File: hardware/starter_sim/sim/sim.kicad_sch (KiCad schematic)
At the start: 22 parts, among them M1 Motor_DC, Q1 AO3400A, Q2 AO3400A, Q3 AO3401A, Q4 AO3400A, Q5 AO3401A, Q6 AO3400A, Q7 AO3401A, Q8 AO3401A

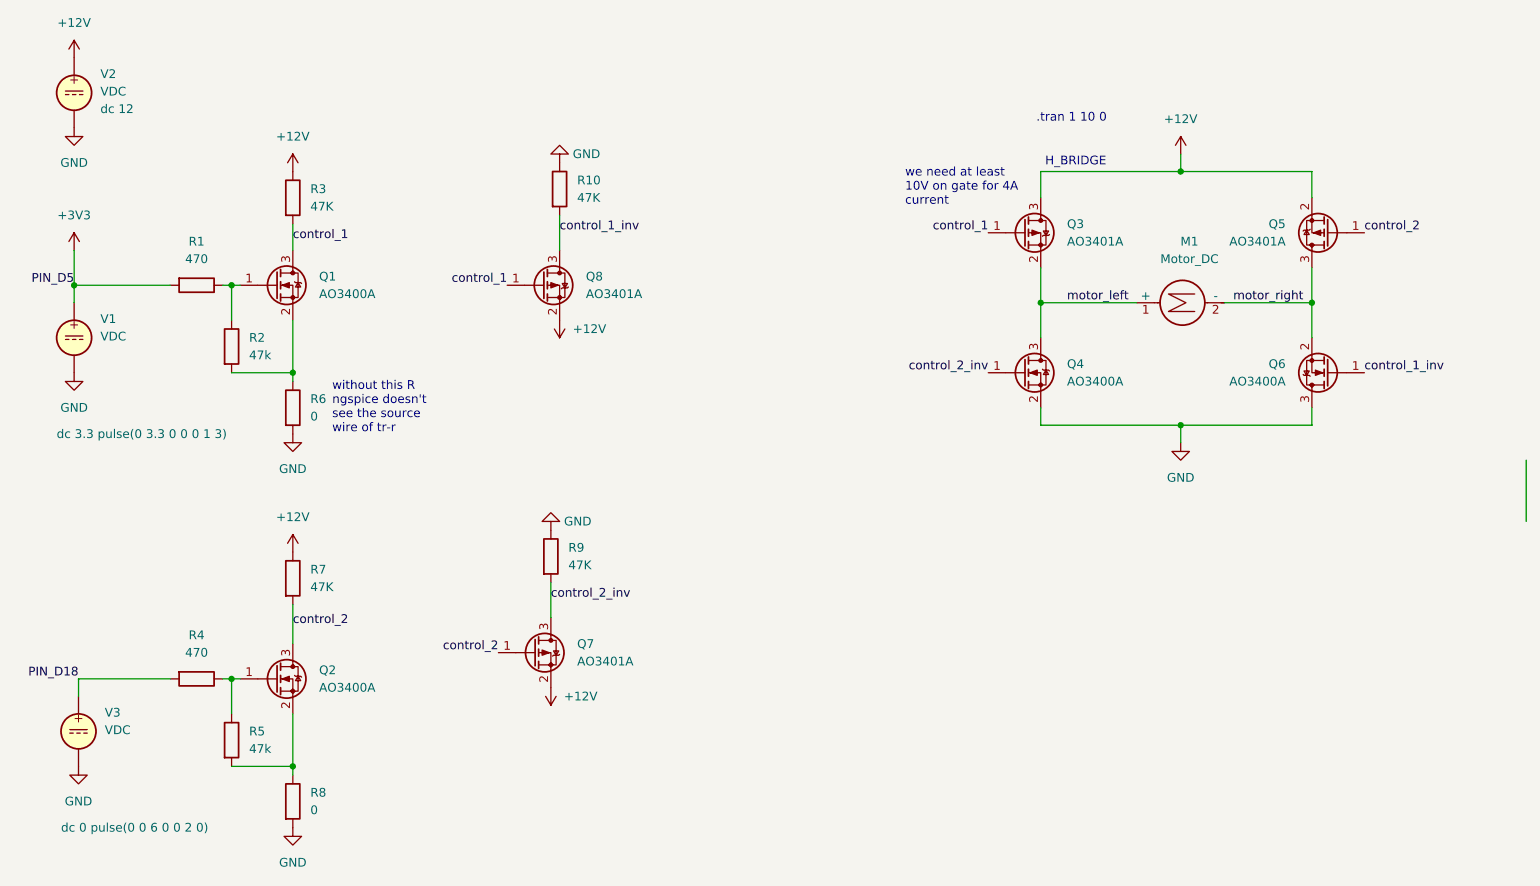
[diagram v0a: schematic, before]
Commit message: wip
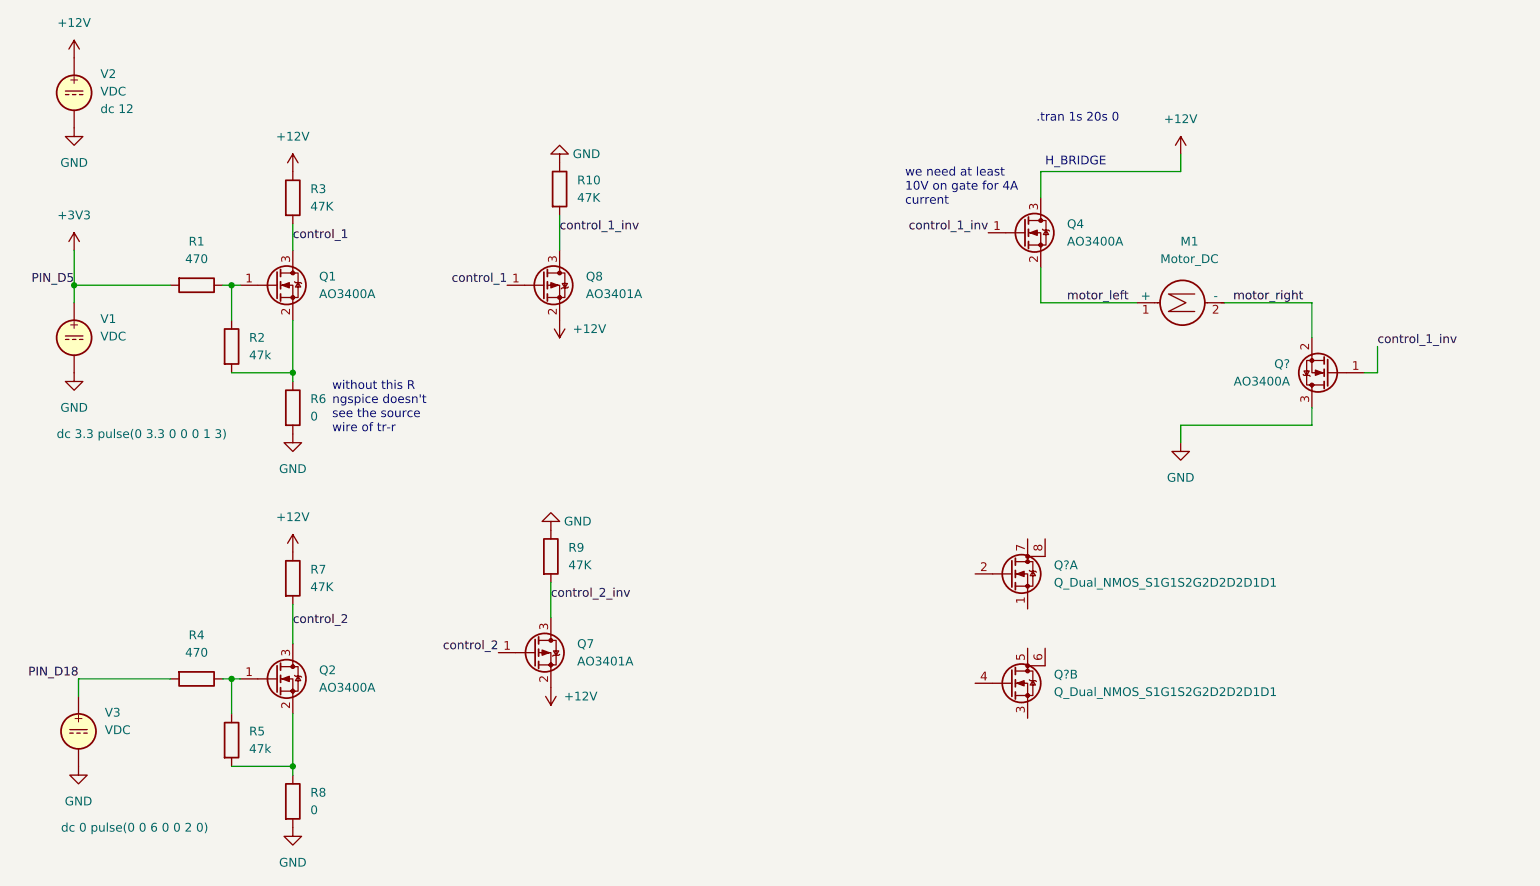
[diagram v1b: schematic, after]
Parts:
- removed Q3, Q5: AO3401A, Package_TO_SOT_SMD:SOT-23, symbol Transistor_FET:AO3401A
- removed Q6: AO3400A, Package_TO_SOT_SMD:SOT-23, symbol Transistor_FET:AO3400A
- added Q? (x2): Q_Dual_NMOS_S1G1S2G2D2D2D1D1, symbol Device:Q_Dual_NMOS_S1G1S2G2D2D2D1D1
- added Q?: AO3400A, Package_TO_SOT_SMD:SOT-23, symbol Transistor_FET:AO3400A
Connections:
- net +12V: now also Q4.3 (D)
- net GND: now also Q?.3 (D); no longer Q4.2 (S)
- net control_1_inv: now also Q4.1 (G), Q?.1 (G)
- net control_2_inv: no longer Q4.1 (G)
- net motor_left: now also Q4.2 (S); no longer Q4.3 (D)
- net motor_right: now also Q?.2 (S)
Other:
- note added: ".tran 1s 20s 0"
- note removed: ".tran 1 10 0"
- moved on the sheet: Q4
